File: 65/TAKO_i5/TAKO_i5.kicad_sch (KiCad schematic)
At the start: 191 parts, among them J3 Conn_01x05, P1 USB_C_Plug_USB2.0, SW1 MX_SW_solder, SW10 MX_SW_solder, SW11 MX_SW_solder, SW12 MX_SW_solder, SW13 MX_SW_solder, SW14 MX_SW_solder, SW15 MX_SW_solder, SW16 MX_SW_solder, SW17 MX_SW_solder, SW18 MX_SW_solder, SW19 MX_SW_solder, SW2 MX_SW_solder, SW20 MX_SW_solder, SW21 MX_SW_solder, SW22 MX_SW_solder, SW23 MX_SW_solder, SW24 MX_SW_solder, SW25 MX_SW_solder, SW26 MX_SW_solder, SW27 MX_SW_solder, SW28 MX_SW_solder, SW29 MX_SW_solder, SW3 MX_SW_solder, SW30 MX_SW_solder, SW31 MX_SW_solder, SW32 RotaryEncoder_Switch, SW33 MX_SW_solder, SW34 MX_SW_solder, SW35 MX_SW_solder, SW36 MX_SW_solder, SW37 MX_SW_solder, SW38 MX_SW_solder, SW39 MX_SW_solder, SW4 MX_SW_solder, SW40 MX_SW_solder, SW41 MX_SW_solder, SW42 MX_SW_solder, SW43 MX_SW_solder, SW44 MX_SW_solder, SW45 MX_SW_solder, SW46 MX_SW_solder, SW47 MX_SW_solder, SW48 RotaryEncoder_Switch, SW49 MX_SW_solder, SW5 MX_SW_solder, SW50 MX_SW_solder, SW51 MX_SW_solder, SW52 MX_SW_solder, SW53 MX_SW_solder, SW54 MX_SW_solder, SW55 MX_SW_solder, SW56 MX_SW_solder, SW57 MX_SW_solder, SW58 MX_SW_solder, SW59 MX_SW_solder, SW6 MX_SW_solder, SW60 MX_SW_solder, SW61 MX_SW_solder, SW62 MX_SW_solder, SW63 MX_SW_solder, SW64 MX_SW_solder, SW65 MX_SW_solder, SW66 MX_SW_solder, SW67 MX_SW_solder, SW68 MX_SW_solder, SW69 MX_SW_solder, SW7 MX_SW_solder, SW70 MX_SW_solder, SW71 MX_SW_solder, SW72 MX_SW_solder, SW73 MX_SW_solder, SW74 MX_SW_solder, SW75 MX_SW_solder, SW76 SW_RESET, SW77 SW_BOOTSEL, SW8 MX_SW_solder, SW9 MX_SW_solder, U1 RP2040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

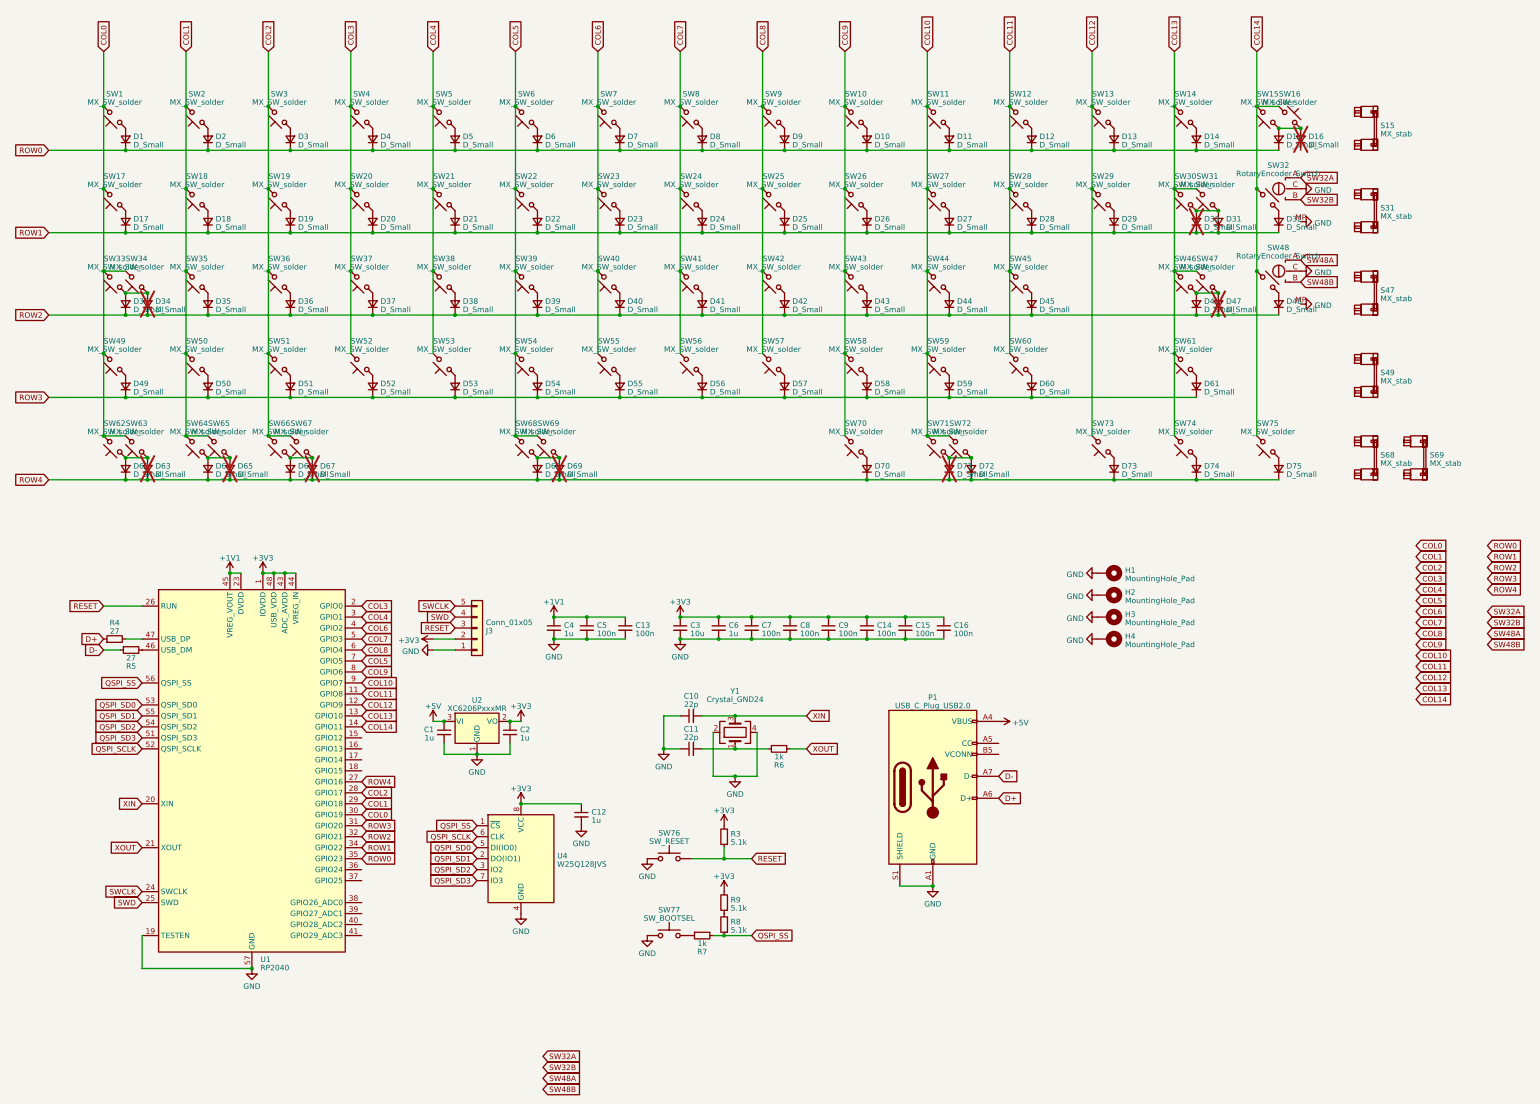
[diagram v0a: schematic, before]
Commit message: uni tako icons
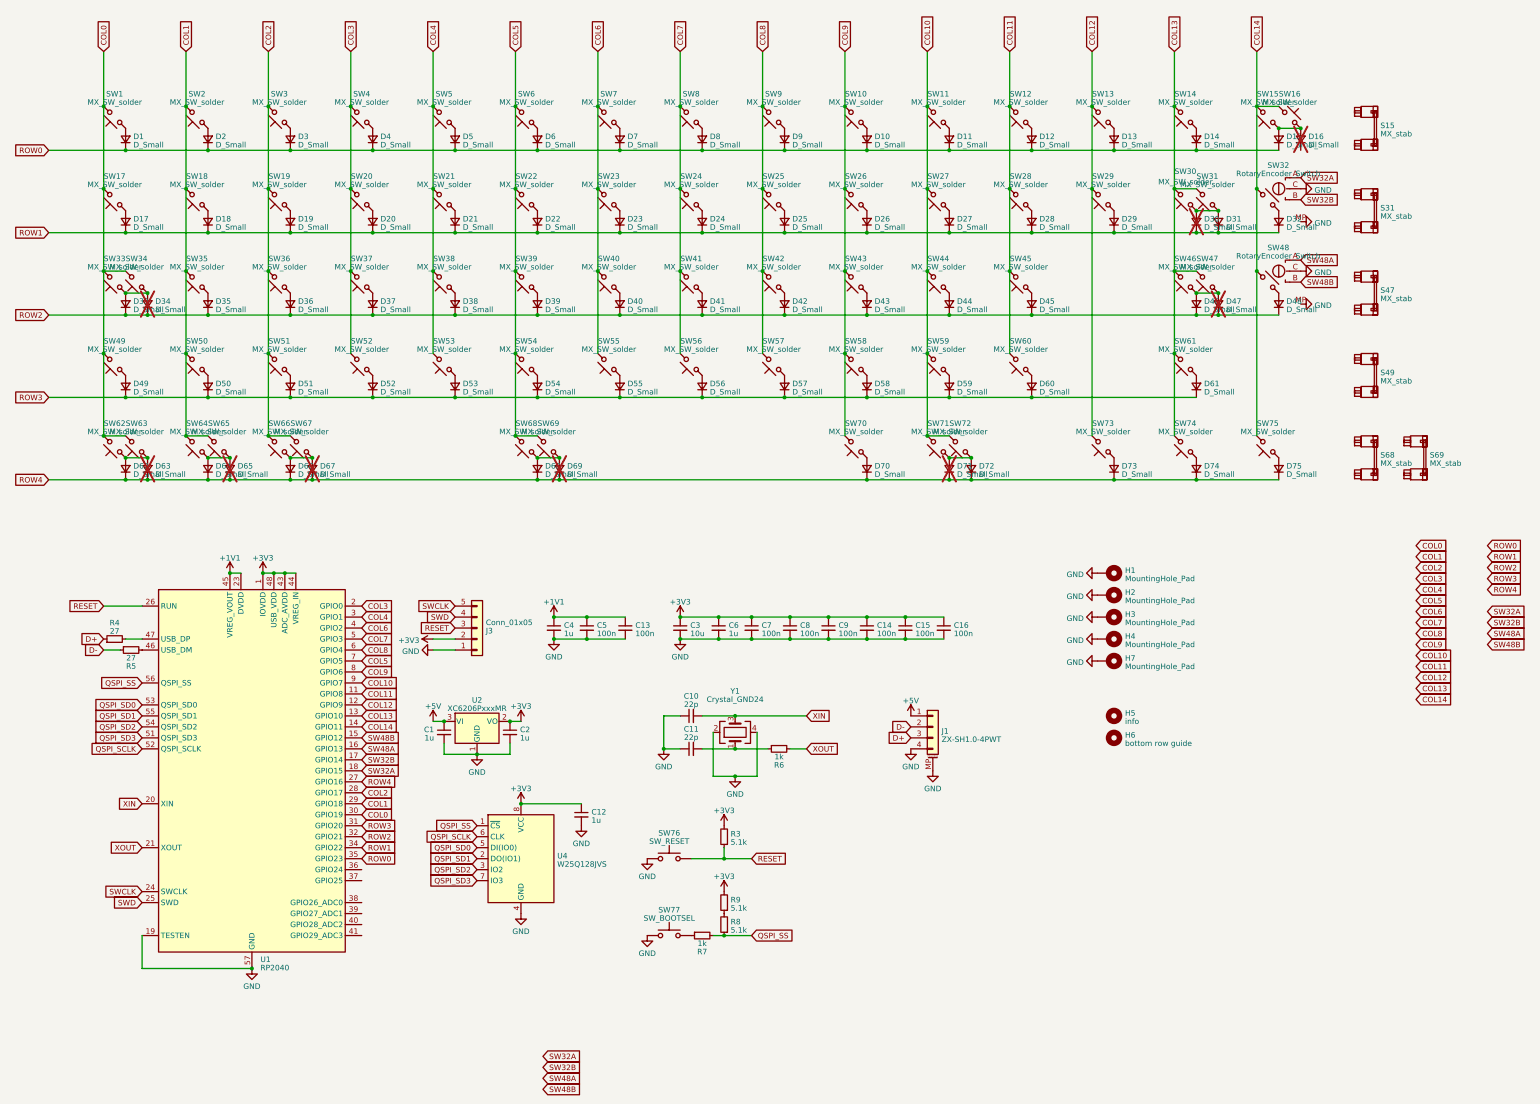
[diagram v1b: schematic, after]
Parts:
- removed P1: USB_C_Plug_USB2.0, Connector_USB:USB_C_Receptacle_HRO_TYPE-C-31-M-12, symbol Connector:USB_C_Plug_USB2.0
- added H5: info, shoonies_parts:info, symbol Mechanical:MountingHole
- added H6: bottom row guide, shoonies_parts:bottom_row_guide, symbol Mechanical:MountingHole
- added H7: MountingHole_Pad, MountingHole:MountingHole_6mm_Pad, symbol Mechanical:MountingHole_Pad
- added J1: ZX-SH1.0-4PWT, Connector_JST:JST_SH_SM04B-SRSS-TB_1x04-1MP_P1.00mm_Horizontal, symbol Connector_Generic_MountingPin:Conn_01x04_MountingPin
- SW1, SW10, SW11, SW12, SW13, SW14, SW15, SW16, SW17, SW18, SW19, SW2, SW20, SW21, SW22, SW23, SW24, SW25, SW26, SW27, SW28, SW29, SW3, SW30, SW31, SW33, SW34, SW35, SW36, SW37, SW38, SW39, SW4, SW40, SW41, SW42, SW43, SW44, SW45, SW46, SW47, SW49, SW5, SW50, SW51, SW52, SW53, SW54, SW55, SW56, SW57, SW58, SW59, SW6, SW60, SW61, SW62, SW63, SW64, SW65, SW66, SW67, SW68, SW69, SW7, SW70, SW71, SW72, SW73, SW74, SW75, SW8, SW9: footprint PCM_marbastlib-mx:SW_MX_HS_1u -> PCM_marbastlib-mx:SW_MX_HS_S_1u
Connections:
- net +5V: now also J1.1 (Pin_1)
- net D+: now also J1.3 (Pin_3)
- net D-: now also J1.2 (Pin_2)
- net GND: now also H7.1, J1.4 (Pin_4), J1.MP (MountPin)
- net SW32A: now also U1.18 (GPIO15)
- net SW32B: now also U1.17 (GPIO14)
- net SW48A: now also U1.16 (GPIO13)
- net SW48B: now also U1.15 (GPIO12)

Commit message: i5v5
split backspace
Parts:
- H5, H6, J3, SW76, SW77: now left out of the parts list
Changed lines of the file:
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@@
   )
   (symbol (lib_id "Mechanical:MountingHole") (at 265.43 179.07 0) (unit 1)
-    (in_bom yes) (on_board yes) (dnp no) (fields_autoplaced)
+    (in_bom no) (on_board yes) (dnp no) (fields_autoplaced)
     (property "Reference" "H5" (at 267.97 178.4263 0)
       (effects (font (size 1.27 1.27)) (justify left))
@@
   )
   (symbol (lib_id "Mechanical:MountingHole") (at 265.43 184.15 0) (unit 1)
-    (in_bom yes) (on_board yes) (dnp no) (fields_autoplaced)
+    (in_bom no) (on_board yes) (dnp no) (fields_autoplaced)
     (property "Reference" "H6" (at 267.97 183.5063 0)
       (effects (font (size 1.27 1.27)) (justify left))
@@
   )
   (symbol (lib_id "Switch:SW_Push") (at 162.56 229.87 0) (unit 1)
-    (in_bom yes) (on_board yes) (dnp no) (fields_autoplaced)
+    (in_bom no) (on_board yes) (dnp no) (fields_autoplaced)
     (property "Reference" "SW77" (at 162.56 223.9391 0)
       (effects (font (size 1.27 1.27)))
@@
   )
   (symbol (lib_id "Connector_Generic:Conn_01x05") (at 118.11 158.75 0) (mirror x) (unit 1)
-    (in_bom yes) (on_board yes) (dnp no)
+    (in_bom no) (on_board yes) (dnp no)
     (property "Reference" "J3" (at 120.142 159.3937 0)
       (effects (font (size 1.27 1.27)) (justify left))
@@
   )
   (symbol (lib_id "Switch:SW_Push") (at 162.56 212.09 0) (unit 1)
-    (in_bom yes) (on_board yes) (dnp no) (fields_autoplaced)
+    (in_bom no) (on_board yes) (dnp no) (fields_autoplaced)
     (property "Reference" "SW76" (at 162.56 206.1591 0)
       (effects (font (size 1.27 1.27)))
